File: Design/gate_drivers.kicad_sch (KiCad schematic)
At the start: 11 parts

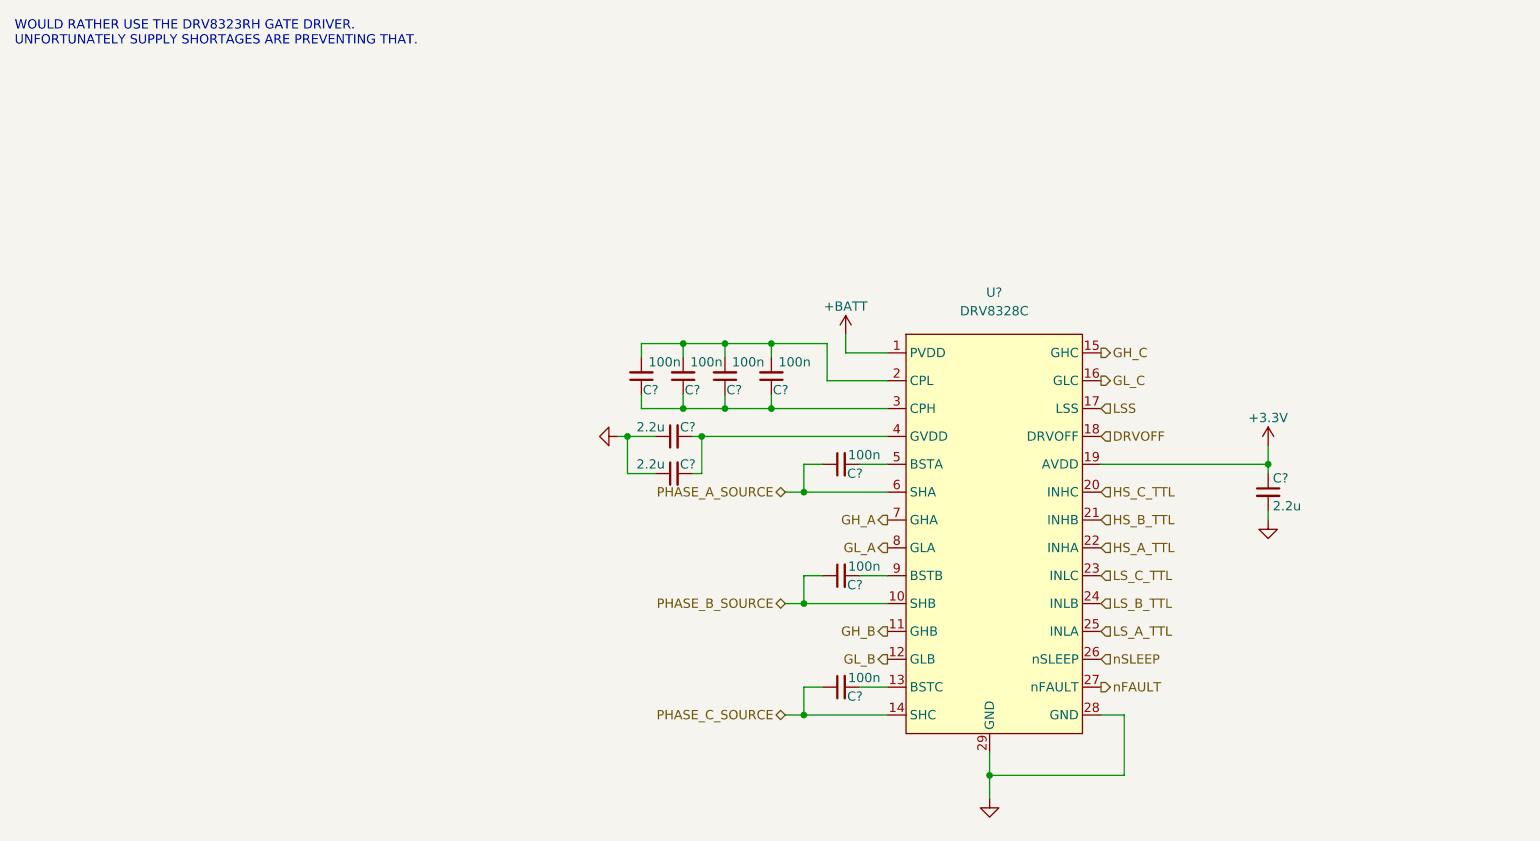
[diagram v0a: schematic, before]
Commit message: drv8323RH
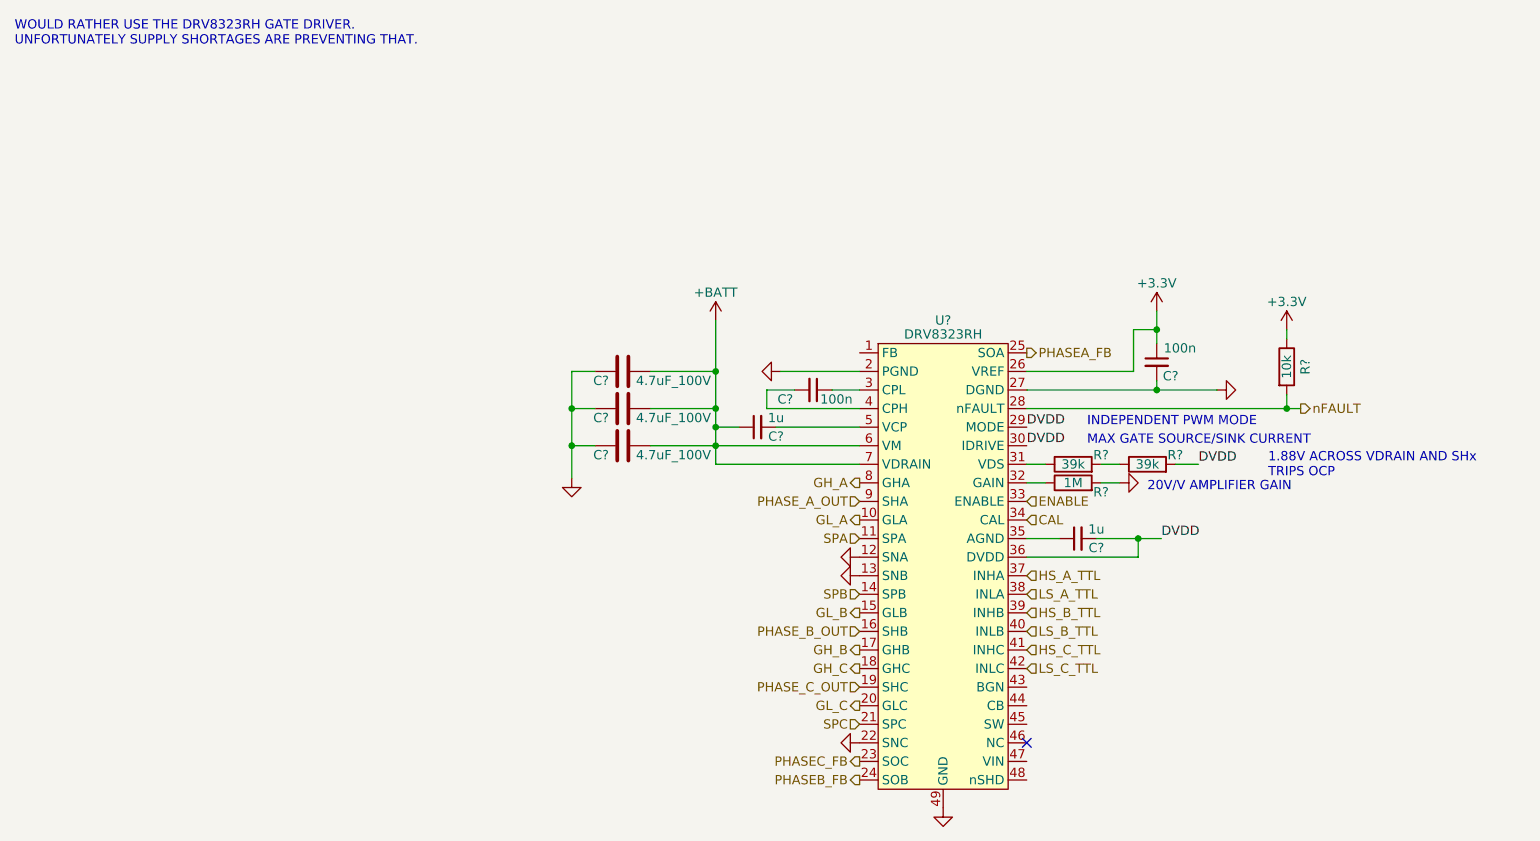
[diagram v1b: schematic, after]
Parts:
- removed C? (x7): 100n, symbol Device:C_Small
- removed C? (x3): 2.2u, symbol Device:C_Small
- removed U?: DRV8328C, symbol TI:DRV8328C
- added C? (x3): 4.7uF_100V, symbol Device:C
- added C? (x2): 100n, symbol Device:C_Small
- added C? (x2): 1u, symbol Device:C_Small
- added R?: 1M, symbol Device:R
- added R?: 10k, symbol Device:R
- added R? (x2): 39k, symbol Device:R
- added U?: DRV8323RH, Package_DFN_QFN:QFN-48-1EP_7x7mm_P0.5mm_EP5.15x5.15mm_ThermalVias, symbol TI:DRV8323RH
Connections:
- net +3.3V: now also C?.1, R?.1, U?.26 (VREF)
- net +BATT: now also C?.1, C?.2, C?.2, C?.2, U?.6 (VM), U?.7 (VDRAIN)
- net GH_A: now also U?.8 (GHA)
- net GH_B: now also U?.17 (GHB)
- net GH_C: now also U?.18 (GHC)
- net GL_A: now also U?.10 (GLA)
- net GL_B: now also U?.15 (GLB)
- net GL_C: now also U?.20 (GLC)
- net GND: now also C?.1, C?.1, C?.1, C?.2, R?.2, U?.12 (SNA), U?.13 (SNB), U?.2 (PGND), U?.22 (SNC), U?.27 (DGND), U?.49 (GND)
- net HS_A_TTL: now also U?.37 (INHA)
- net HS_B_TTL: now also U?.39 (INHB)
- net HS_C_TTL: now also U?.41 (INHC)
- net LS_A_TTL: now also U?.38 (INLA)
- net LS_B_TTL: now also U?.40 (INLB)
- net LS_C_TTL: now also U?.42 (INLC)
- net nFAULT: now also R?.2, U?.28 (nFAULT)
- new net: R?.1, U?.32 (GAIN)
- new net: R?.1, U?.31 (VDS)
- new net: R?.1, R?.2
- new net: C?.2, U?.5 (VCP)
- new net: C?.1, U?.3 (CPL)
- new net: C?.2, U?.4 (CPH)
- new net: C?.1, U?.35 (AGND)
- new net CAL: U?.34 (CAL)
- new net DVDD: C?.2, R?.2, U?.29 (MODE), U?.30 (IDRIVE), U?.36 (DVDD)
- new net ENABLE: U?.33 (ENABLE)
- new net PHASEA_FB: U?.25 (SOA)
- new net PHASEB_FB: U?.24 (SOB)
- new net PHASEC_FB: U?.23 (SOC)
- new net PHASE_A_OUT: U?.9 (SHA)
- new net PHASE_B_OUT: U?.16 (SHB)
- new net PHASE_C_OUT: U?.19 (SHC)
- new net SPA: U?.11 (SPA)
- new net SPB: U?.14 (SPB)
- new net SPC: U?.21 (SPC)
- no-connect marks 0 -> 1
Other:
- note added: "1.88V ACROSS VDRAIN AND SHx TRIPS OCP"
- note added: "20V/V AMPLIFIER GAIN"
- note added: "INDEPENDENT PWM MODE"
- note added: "MAX GATE SOURCE/SINK CURRENT"
